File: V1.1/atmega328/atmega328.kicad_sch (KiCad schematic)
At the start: 17 parts

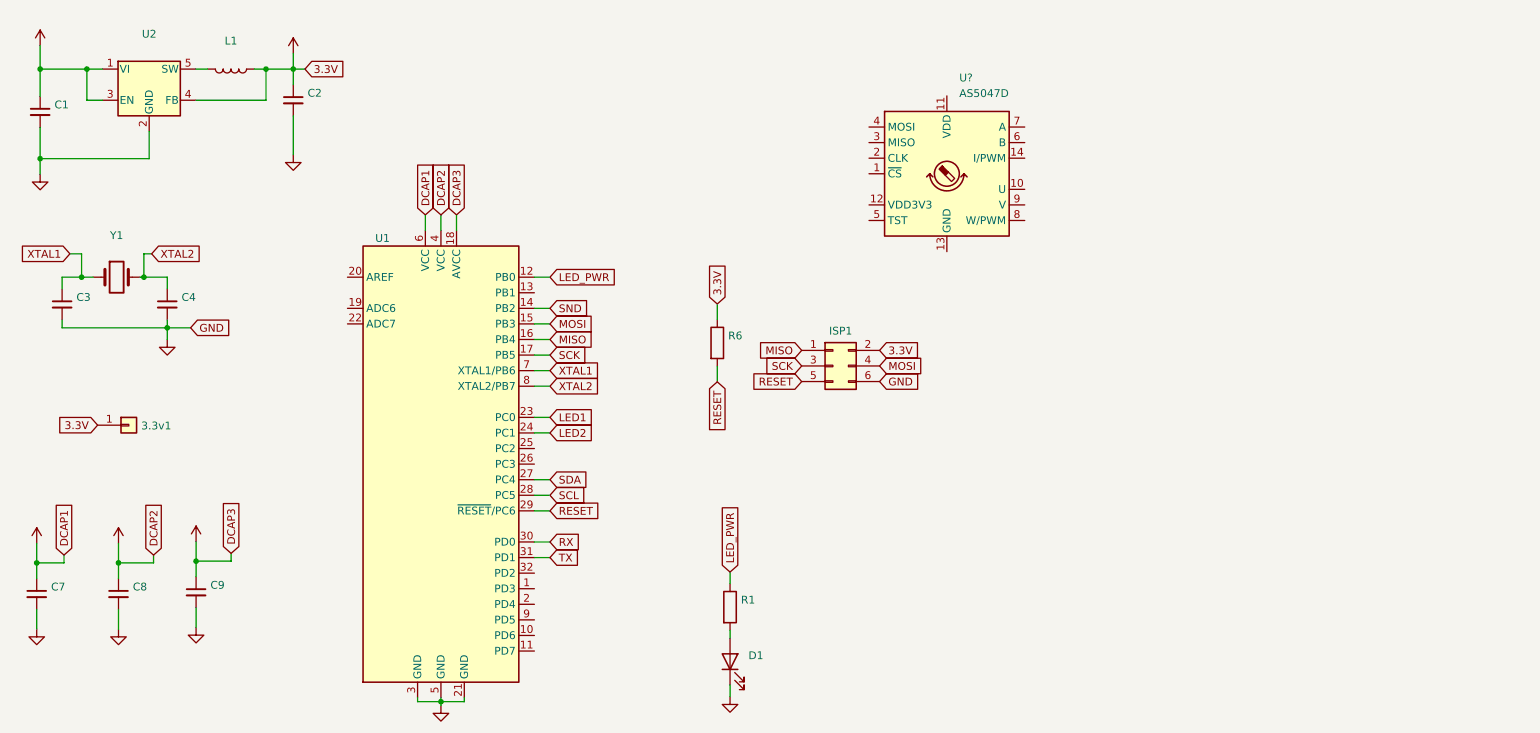
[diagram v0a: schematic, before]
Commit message: things
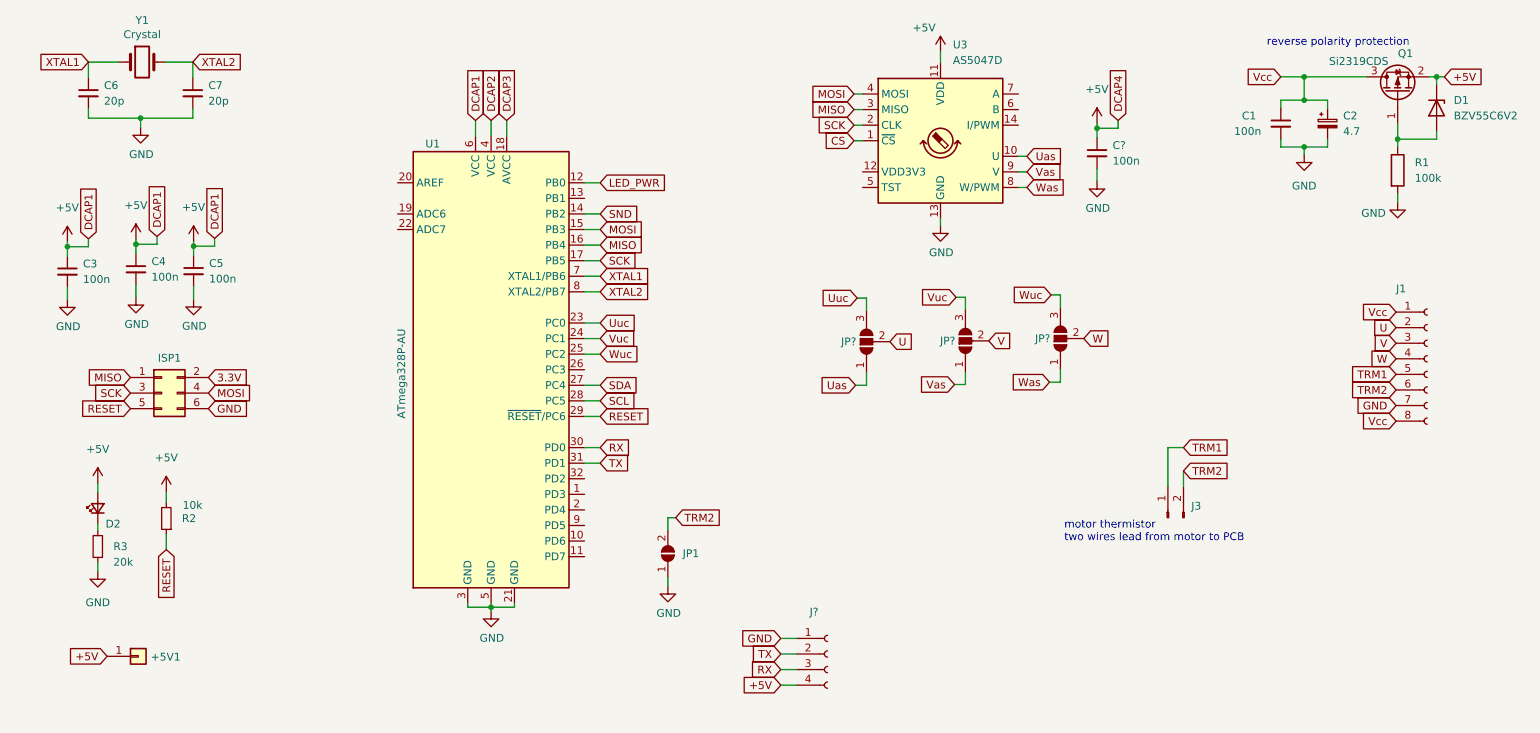
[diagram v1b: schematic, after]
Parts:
- removed C2, C8, C9: (no value), symbol Device:C_Small
- removed D1: (no value), symbol Device:LED
- removed L1: (no value), symbol Device:L
- removed R6: (no value), symbol Device:R
- removed U2: (no value), symbol Regulator_Switching:TPS62203DBV
- added C2: 4.7, Capacitor_Tantalum_SMD:CP_EIA-3216-18_Kemet-A, symbol Device:C_Polarized_Small
- added C5, C?: 100n, Capacitor_SMD:C_0402_1005Metric, symbol Device:C_Small
- added C6: 20p, Capacitor_SMD:C_0402_1005Metric, symbol Device:C_Small
- added D1: BZV55C6V2, Diode_SMD:D_MiniMELF, symbol Diode:BZV55B10
- added D2: RED_LED, LED_SMD:LED_0603_1608Metric, symbol Device:LED_Small
- added J1: Conn_01x08_Female, Connector_PinSocket_2.54mm:PinSocket_1x08_P2.54mm_Vertical, symbol Connector:Conn_01x08_Female
- added J3: Conn_01x02_Male, Connector_PinHeader_2.54mm:PinHeader_1x02_P2.54mm_Vertical, symbol Connector:Conn_01x02_Male
- added J?: Conn_01x04_Female, Connector_PinSocket_2.54mm:PinSocket_1x04_P2.54mm_Vertical, symbol Connector:Conn_01x04_Female
- added JP1: SolderJumper_2_Open, Jumper:SolderJumper-2_P1.3mm_Open_Pad1.0x1.5mm, symbol Jumper:SolderJumper_2_Open
- added JP? (x3): SolderJumper_3_Open, Jumper:SolderJumper-3_P1.3mm_Open_RoundedPad1.0x1.5mm_NumberLabels, symbol Jumper:SolderJumper_3_Open
- added Q1: Si2319CDS, Package_TO_SOT_SMD:SOT-23, symbol Transistor_FET:Si2319CDS
- added R2: 10k, Resistor_SMD:R_0603_1608Metric, symbol Device:R_Small
- added R3: 20k, Resistor_SMD:R_0603_1608Metric, symbol Device:R_Small
- +5V1: renamed from 3.3v1; value (none) -> Conn_01x01; footprint (none) -> Connector_PinHeader_2.54mm:PinHeader_1x01_P2.54mm_Vertical
- C1: value (none) -> 100n; footprint (none) -> Capacitor_SMD:C_0603_1608Metric; LCSC (none) -> C346191
- C3, C4: value (none) -> 100n; footprint (none) -> Capacitor_SMD:C_0402_1005Metric; LCSC (none) -> C1525
- C7: value (none) -> 20p; footprint (none) -> Capacitor_SMD:C_0402_1005Metric; LCSC (none) -> C880615
- ISP1: value (none) -> Conn_02x03_Top_Bottom; footprint (none) -> Connector_PinSocket_2.54mm:isp_6pin
- R1: value (none) -> 100k; footprint (none) -> Resistor_SMD:R_0603_1608Metric; LCSC (none) -> C14675
- U1: value (none) -> ATmega328P-AU; footprint (none) -> Package_QFP:TQFP-32_7x7mm_P0.8mm
- Y1: value (none) -> Crystal; footprint (none) -> Crystal:Crystal_SMD_5032-2Pin_5.0x3.2mm; LCSC (none) -> C122521
- gave numbers to parts that had none: 1
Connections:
- net GND: now also R1.2, U3.13 (GND), C2.2, C5.2, C6.2, C?.2, J1.7 (Pin_7), J?.1 (Pin_1), JP1.1 (A), R3.1
- net LED_PWR: no longer R1.1
- net MISO: now also U3.3 (MISO)
- net MOSI: now also U3.4 (MOSI)
- net RESET: now also R2.1
- net RX: now also J?.3 (Pin_3)
- net SCK: now also U3.2 (CLK)
- net TX: now also J?.2 (Pin_2)
- net XTAL1: now also C6.1; no longer C3.1
- net XTAL2: now also C7.1; no longer C4.1
- net Wuc: now reaches U1.25 (PC2)
- net Wuc: now also JP?.3 (B)
- net CS: now reaches U3.1 (~{CS})
- net Uas: now reaches U3.10 (U)
- net Uas: now also JP?.1 (A)
- net +5V: now reaches U3.11 (VDD)
- net +5V: now also +5V1.1 (Pin_1), C3.1, C4.1, U1.6 (VCC), C5.1, C?.1, D1.1 (K), D2.2 (A), J?.4 (Pin_4), Q1.2 (S), R2.2
- net Was: now reaches U3.8 (W/PWM)
- net Was: now also JP?.1 (A)
- net Vas: now reaches U3.9 (V)
- net Vas: now also JP?.1 (A)
- removed net +3V3: +5V1.1 (Pin_1), C7.1, ISP1.2 (Pin_2), U1.18 (AVCC), U1.4 (VCC), U1.6 (VCC)
- net LED1 renamed Uuc
- net Uuc: now also JP?.3 (B)
- net LED2 renamed Vuc
- net Vuc: now also JP?.3 (B)
- net VCC renamed Vcc
- net Vcc: now also C2.1, J1.1 (Pin_1), J1.8 (Pin_8), Q1.3 (D)
- new net: D1.2 (A), Q1.1 (G), R1.1
- new net: D2.1 (K), R3.2
- new net 3.3V: ISP1.2 (Pin_2)
- new net DCAP2: U1.4 (VCC)
- new net DCAP3: U1.18 (AVCC)
- new net TRM1: J1.5 (Pin_5), J3.1 (Pin_1)
- new net TRM2: J1.6 (Pin_6), J3.2 (Pin_2), JP1.2 (B)
- new net U: J1.2 (Pin_2), JP?.2 (C)
- new net V: J1.3 (Pin_3), JP?.2 (C)
- new net W: J1.4 (Pin_4), JP?.2 (C)
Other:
- note added: "motor thermistor two wires lead from motor to PCB"
- note added: "reverse polarity protection"
- moved on the sheet: +5V1, ISP1, U1, U3, Y1
